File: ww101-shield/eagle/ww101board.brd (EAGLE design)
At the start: 59.1 x 64.6 mm, 58 parts

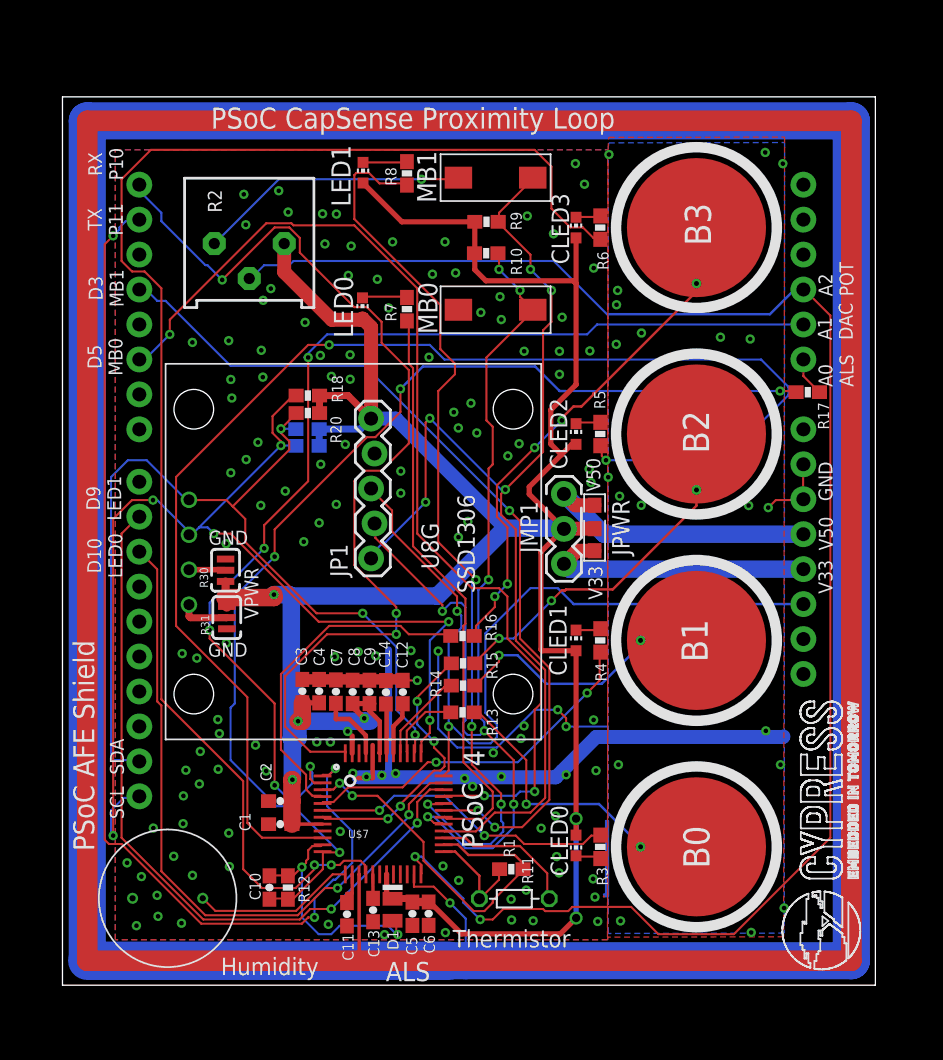
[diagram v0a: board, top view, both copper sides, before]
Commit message: Right before autoroute
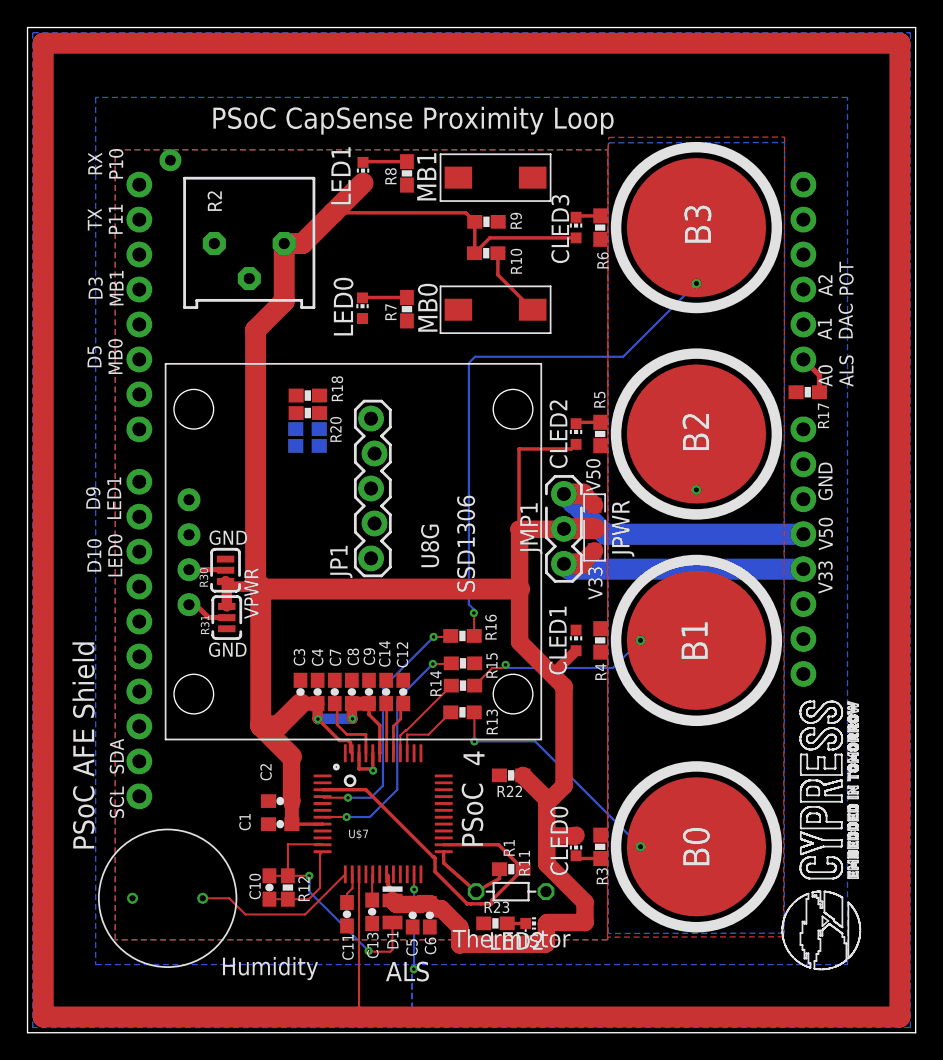
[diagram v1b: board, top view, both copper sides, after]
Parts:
- added LED2: red, adafruit:CHIP-LED0603
- added R22: 10K, PatternAgents-ProtoPads:0603-RES
- added R23: 560, PatternAgents-ProtoPads:0603-RES
- moved R11 0.56 mm to (29.5, 3.24)
- moved C3 0.15 mm to (14.2, 17.8)
- moved C6 0.15 mm to (23.6, 1.52)
- moved C13 0.14 mm to (19.4, 1.78)
- moved D1 0.13 mm to (20.9, 3.10)
- moved C4 0.12 mm to (15.5, 17.8)
- moved C5 0.11 mm to (22.4, 1.52)
- moved C7 0.09 mm to (16.7, 17.8)
- moved C8 0.06 mm to (18.0, 17.8)
- renumbered MB0 to MB2
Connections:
- net MBLED1 renamed LED1
- removed net D10: U$1.D10, U$7.35
- removed net D3: U$1.D3, U$7.31
- removed net D9: U$1.D9, U$7.34
- removed net MB0: JP1.2, MB2.P$2, R10.2, U$7.29
- removed net MBLED0: R7.1, U$7.30
- new net D11: U$1.D11, U$7.35
- new net D12: U$1.D12, U$7.30
- new net D13: U$1.D13, U$7.21
- new net D4: U$1.D4, U$7.31
- new net FUTUREARD: U$1.D2, U$7.22
- new net LED2: R7.1, U$7.34
- new net MB2: JP1.1, MB2.P$2, R10.2, U$7.28
- new net N$3: LED2.C, R23.2
- new net PROXLED: R23.1, U$7.20
- net MB1: now also JP1.2, U$7.29; no longer JP1.1, U$7.28
- net VPWR: now also LED2.A, R22.1
- net XRES: now also R22.2
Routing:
- net CSHIELD: track 241.8 -> 6.92 mm, vias 1 -> 2
- net GND: track 129.0 -> 3.47 mm, vias 151 -> 2
- net POT: track 122.0 -> 0.00 mm, vias 2 -> 0
- net CBLED3: track 105.8 -> 0.00 mm, vias 2 -> 0
- net CBLED2: track 100.0 -> 0.00 mm, vias 2 -> 0
- net SCL: track 81.4 -> 0.00 mm, vias 6 -> 0
- net VDAC: track 80.3 -> 0.00 mm, vias 5 -> 0
- net UARTRX: track 78.8 -> 0.00 mm, vias 3 -> 0
- net MB1: track 78.6 -> 0.00 mm, vias 5 -> 0
- net MB0: track 76.2 -> 0.00 mm, vias 7 -> 0
- net D5: track 75.3 -> 0.00 mm, vias 3 -> 0
- net TIA_OUT: track 80.8 -> 6.73 mm, vias 4 -> 0
- net UARTTX: track 71.6 -> 0.00 mm, vias 3 -> 0
- net SDA: track 69.1 -> 0.00 mm, vias 3 -> 0
- net LED1: track 66.2 -> 0.00 mm, vias 4 -> 0
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- added copper zone on layer 16, net CSHIELD
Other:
- board size 59.1 x 64.6 mm -> 64.5 x 73.1 mm
